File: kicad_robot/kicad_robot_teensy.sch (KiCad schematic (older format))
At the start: 21 parts, among them Q1 IRLML0030, U12->5 R-78E5.0-1.0

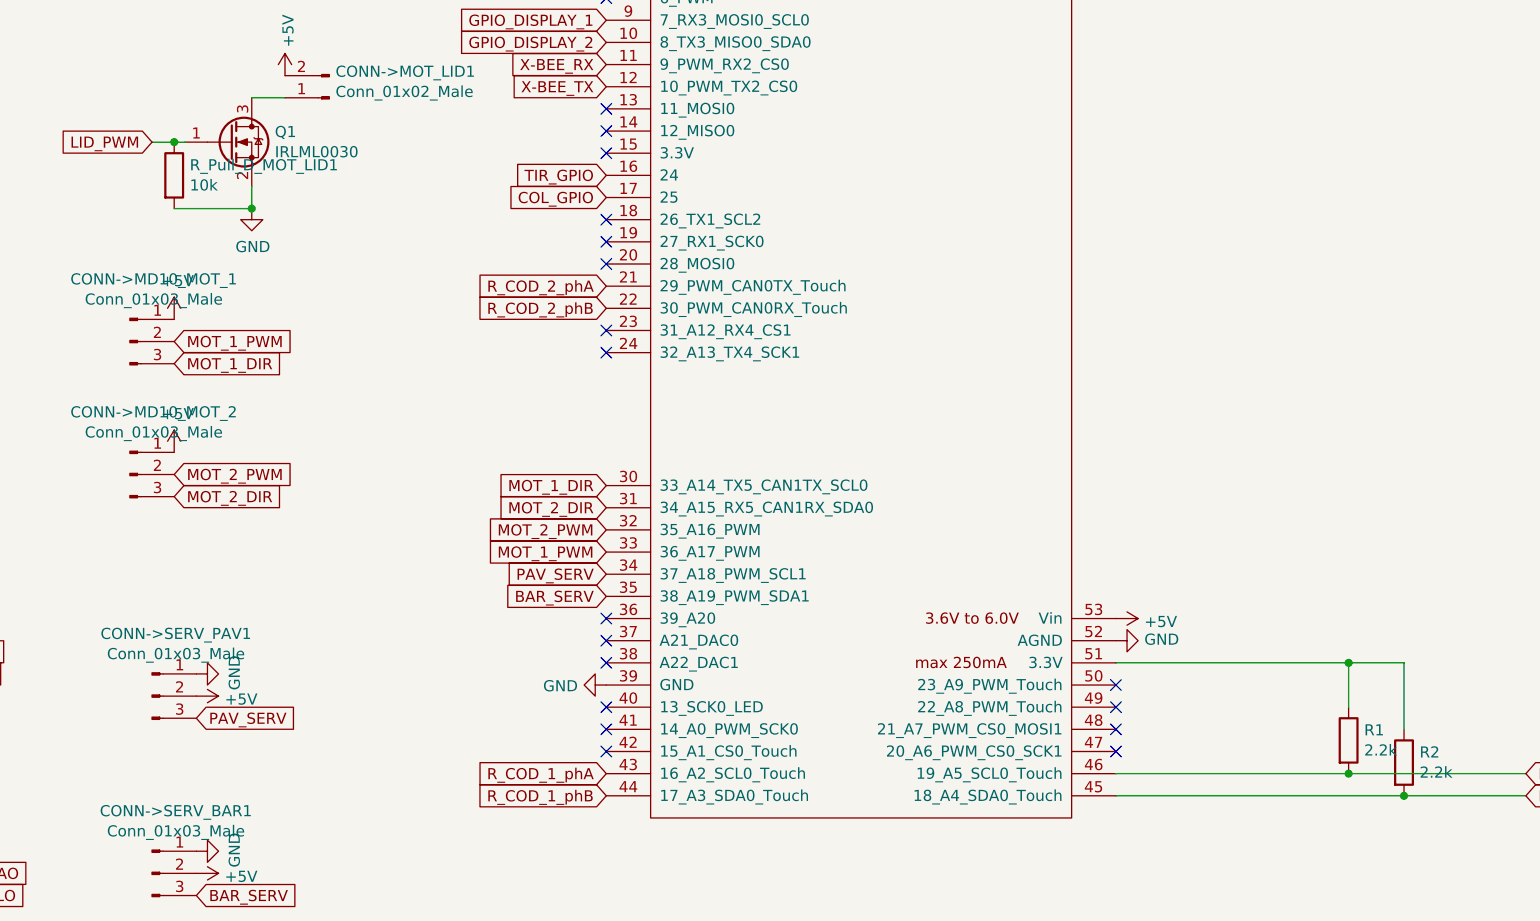
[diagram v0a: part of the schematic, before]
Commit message: Carte Teensy V2.0
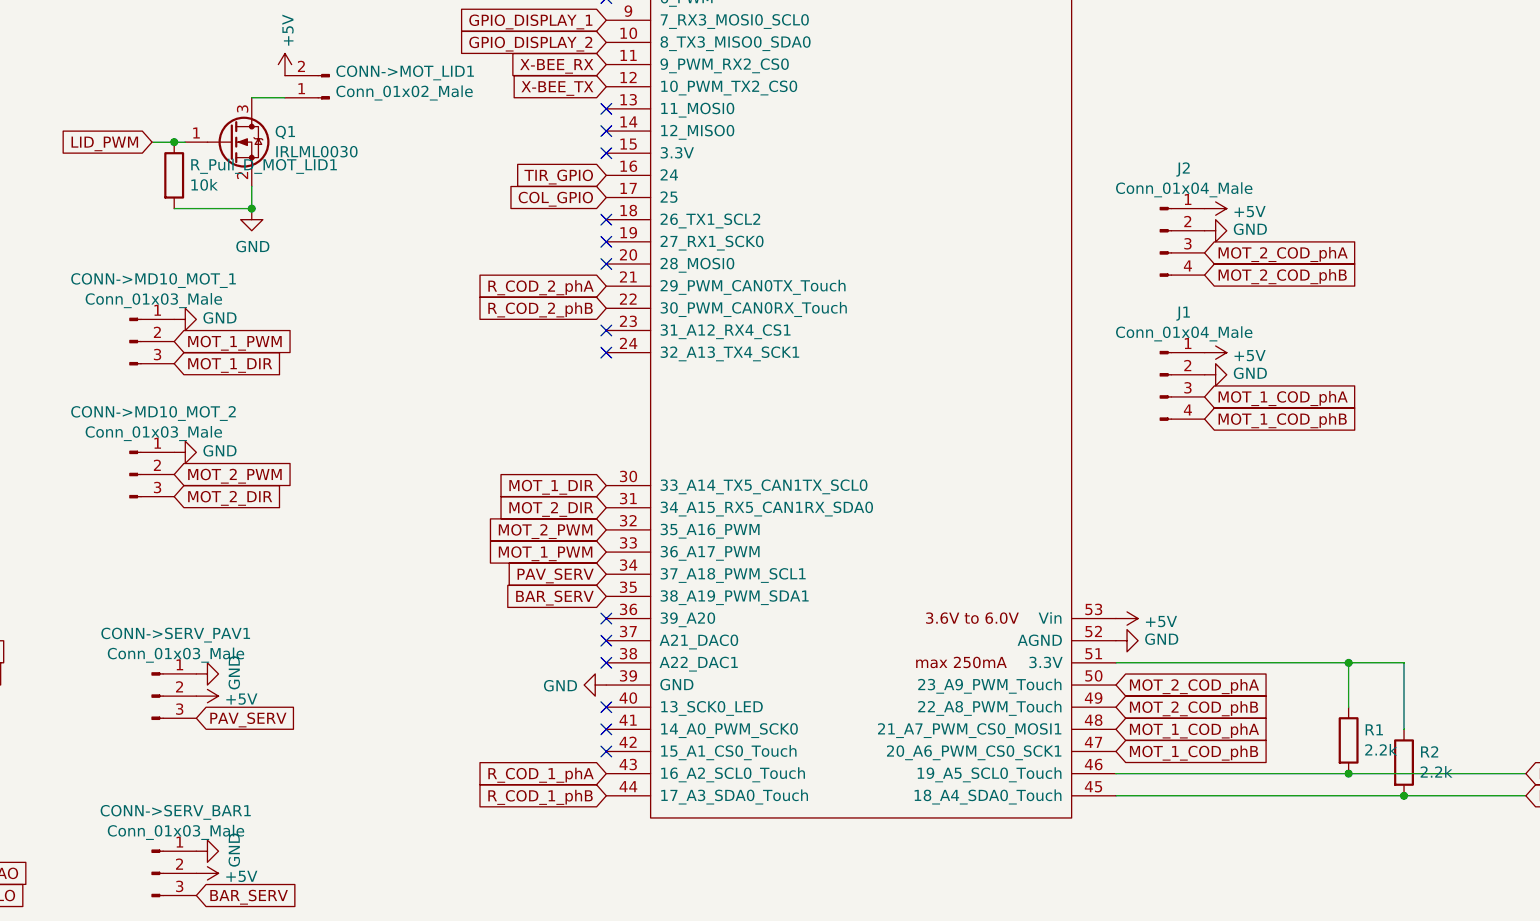
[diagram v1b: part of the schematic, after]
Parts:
- added J1, J2: Conn_01x04_Male, symbol Connector:Conn_01x04_Male
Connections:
- net +5V: now also J1.1 (Pin_1), J2.1 (Pin_1); no longer CONN->MD10_MOT_1.1 (Pin_1), CONN->MD10_MOT_2.1 (Pin_1)
- net GND: now also CONN->MD10_MOT_1.1 (Pin_1), CONN->MD10_MOT_2.1 (Pin_1), J1.2 (Pin_2), J2.2 (Pin_2)
- net MOT_1_COD_phB: now reaches CARTE_MICR_COTROL1.47 (20_A6_PWM_CS0_SCK1)
- net MOT_1_COD_phB: now also J1.4 (Pin_4)
- net MOT_1_COD_phA: now reaches CARTE_MICR_COTROL1.48 (21_A7_PWM_CS0_MOSI1)
- net MOT_1_COD_phA: now also J1.3 (Pin_3)
- net MOT_2_COD_phB: now reaches CARTE_MICR_COTROL1.49 (22_A8_PWM_Touch)
- net MOT_2_COD_phB: now also J2.4 (Pin_4)
- net MOT_2_COD_phA: now reaches CARTE_MICR_COTROL1.50 (23_A9_PWM_Touch)
- net MOT_2_COD_phA: now also J2.3 (Pin_3)
- no-connect marks 22 -> 18
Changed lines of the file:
@@
 NoConn ~ 4100 5600
 NoConn ~ 4100 5700
-NoConn ~ 6400 5700
-NoConn ~ 6400 5600
-NoConn ~ 6400 5500
-NoConn ~ 6400 5400
 $Comp
 L power:GND #PWR0103
@@
 MOT_1_PWM
 $Comp
-L power:+5V #PWR0123
-U 1 1 603CB818
-P 2150 3750
-F 0 "#PWR0123" H 2150 3600 50  0001 C CNN
-F 1 "+5V" H 2165 3923 50  0000 C CNN
-F 2 "" H 2150 3750 50  0001 C CNN
-F 3 "" H 2150 3750 50  0001 C CNN
-	1    2150 3750
-	1    0    0    -1
-$EndComp
-$Comp
 L Connector:Conn_01x03_Male CONN->MD10_MOT_2
 U 1 1 603CCE1B
@@
 	1    0    0    -1
 $EndComp
-$Comp
-L power:+5V #PWR0124
-U 1 1 603CCE23
-P 2150 4350
-F 0 "#PWR0124" H 2150 4200 50  0001 C CNN
-F 1 "+5V" H 2165 4523 50  0000 C CNN
-F 2 "" H 2150 4350 50  0001 C CNN
-F 3 "" H 2150 4350 50  0001 C CNN
-	1    2150 4350
-	1    0    0    -1
-$EndComp
 Text GLabel 2150 4450 2    50   Input ~ 0
 MOT_2_PWM
@@
 Wire Wire Line
 	6400 5300 7450 5300
+$Comp
+L power:GND #PWR03
+U 1 1 6040DF36
+P 2150 3750
+F 0 "#PWR03" H 2150 3500 50  0001 C CNN
+F 1 "GND" V 2155 3622 50  0000 R CNN
+F 2 "" H 2150 3750 50  0001 C CNN
+F 3 "" H 2150 3750 50  0001 C CNN
+	1    2150 3750
+	0    -1   -1   0
+$EndComp
+$Comp
+L power:GND #PWR04
+U 1 1 6040E309
+P 2150 4350
+F 0 "#PWR04" H 2150 4100 50  0001 C CNN
+F 1 "GND" V 2155 4222 50  0000 R CNN
+F 2 "" H 2150 4350 50  0001 C CNN
+F 3 "" H 2150 4350 50  0001 C CNN
+	1    2150 4350
+	0    -1   -1   0
+$EndComp
+$Comp
+L Connector:Conn_01x04_Male J1
+U 1 1 6040EEA7
+P 6600 4000
+F 0 "J1" H 6708 4281 50  0000 C CNN
+F 1 "Conn_01x04_Male" H 6708 4190 50  0000 C CNN
+F 2 "" H 6600 4000 50  0001 C CNN
+F 3 "~" H 6600 4000 50  0001 C CNN
+	1    6600 4000
+	1    0    0    -1
+$EndComp
+$Comp
+L power:GND #PWR02
+U 1 1 6040FE4E
+P 6800 4000
+F 0 "#PWR02" H 6800 3750 50  0001 C CNN
+F 1 "GND" V 6805 3872 50  0000 R CNN
+F 2 "" H 6800 4000 50  0001 C CNN
+F 3 "" H 6800 4000 50  0001 C CNN
+	1    6800 4000
+	0    -1   -1   0
+$EndComp
+$Comp
+L power:+5V #PWR01
+U 1 1 604102FD
+P 6800 3900
+F 0 "#PWR01" H 6800 3750 50  0001 C CNN
+F 1 "+5V" V 6815 4028 50  0000 L CNN
+F 2 "" H 6800 3900 50  0001 C CNN
+F 3 "" H 6800 3900 50  0001 C CNN
+	1    6800 3900
+	0    1    1    0
+$EndComp
+Text GLabel 6800 4100 2    50   Input ~ 0
+MOT_1_COD_phA
+Text GLabel 6800 4200 2    50   Input ~ 0
+MOT_1_COD_phB
+$Comp
+L Connector:Conn_01x04_Male J2
+U 1 1 604159FA
+P 6600 3350
+F 0 "J2" H 6708 3631 50  0000 C CNN
+F 1 "Conn_01x04_Male" H 6708 3540 50  0000 C CNN
+F 2 "" H 6600 3350 50  0001 C CNN
+F 3 "~" H 6600 3350 50  0001 C CNN
+	1    6600 3350
+	1    0    0    -1
+$EndComp
+$Comp
+L power:GND #PWR06
+U 1 1 60415A00
+P 6800 3350
+F 0 "#PWR06" H 6800 3100 50  0001 C CNN
+F 1 "GND" V 6805 3222 50  0000 R CNN
+F 2 "" H 6800 3350 50  0001 C CNN
+F 3 "" H 6800 3350 50  0001 C CNN
+	1    6800 3350
+	0    -1   -1   0
+$EndComp
+$Comp
+L power:+5V #PWR05
+U 1 1 60415A06
+P 6800 3250
+F 0 "#PWR05" H 6800 3100 50  0001 C CNN
+F 1 "+5V" V 6815 3378 50  0000 L CNN
+F 2 "" H 6800 3250 50  0001 C CNN
+F 3 "" H 6800 3250 50  0001 C CNN
+	1    6800 3250
+	0    1    1    0
+$EndComp
+Text GLabel 6800 3450 2    50   Input ~ 0
+MOT_2_COD_phA
+Text GLabel 6800 3550 2    50   Input ~ 0
+MOT_2_COD_phB
+Text GLabel 6400 5400 2    50   Input ~ 0
+MOT_2_COD_phA
+Text GLabel 6400 5500 2    50   Input ~ 0
+MOT_2_COD_phB
+Text GLabel 6400 5600 2    50   Input ~ 0
+MOT_1_COD_phA
+Text GLabel 6400 5700 2    50   Input ~ 0
+MOT_1_COD_phB
 $EndSCHEMATC

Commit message: Teensy V2.1: Carte presque prête
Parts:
- J1, J2: footprint (none) -> Connector_JST:JST_XH_B4B-XH-A_1x04_P2.50mm_Vertical
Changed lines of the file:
@@
 F 0 "J1" H 6708 4281 50  0000 C CNN
 F 1 "Conn_01x04_Male" H 6708 4190 50  0000 C CNN
-F 2 "" H 6600 4000 50  0001 C CNN
+F 2 "Connector_JST:JST_XH_B4B-XH-A_1x04_P2.50mm_Vertical" H 6600 4000 50  0001 C CNN
 F 3 "~" H 6600 4000 50  0001 C CNN
 	1    6600 4000
@@
 F 0 "J2" H 6708 3631 50  0000 C CNN
 F 1 "Conn_01x04_Male" H 6708 3540 50  0000 C CNN
-F 2 "" H 6600 3350 50  0001 C CNN
+F 2 "Connector_JST:JST_XH_B4B-XH-A_1x04_P2.50mm_Vertical" H 6600 3350 50  0001 C CNN
 F 3 "~" H 6600 3350 50  0001 C CNN
 	1    6600 3350
